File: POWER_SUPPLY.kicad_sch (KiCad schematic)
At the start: 70 parts, among them J1 Jack-DC, Q1 NTJD4401NT1G, Q2 NTJD4401NT1G, Q3 NTJD4401NT1G, U20 74LVC1G08, U21 74LVC1G08, U22 LM397, U23 74LVC1G17, U5 LM66100DCK, U6 LMR33640ADDA, U7 LMR33640ADDA

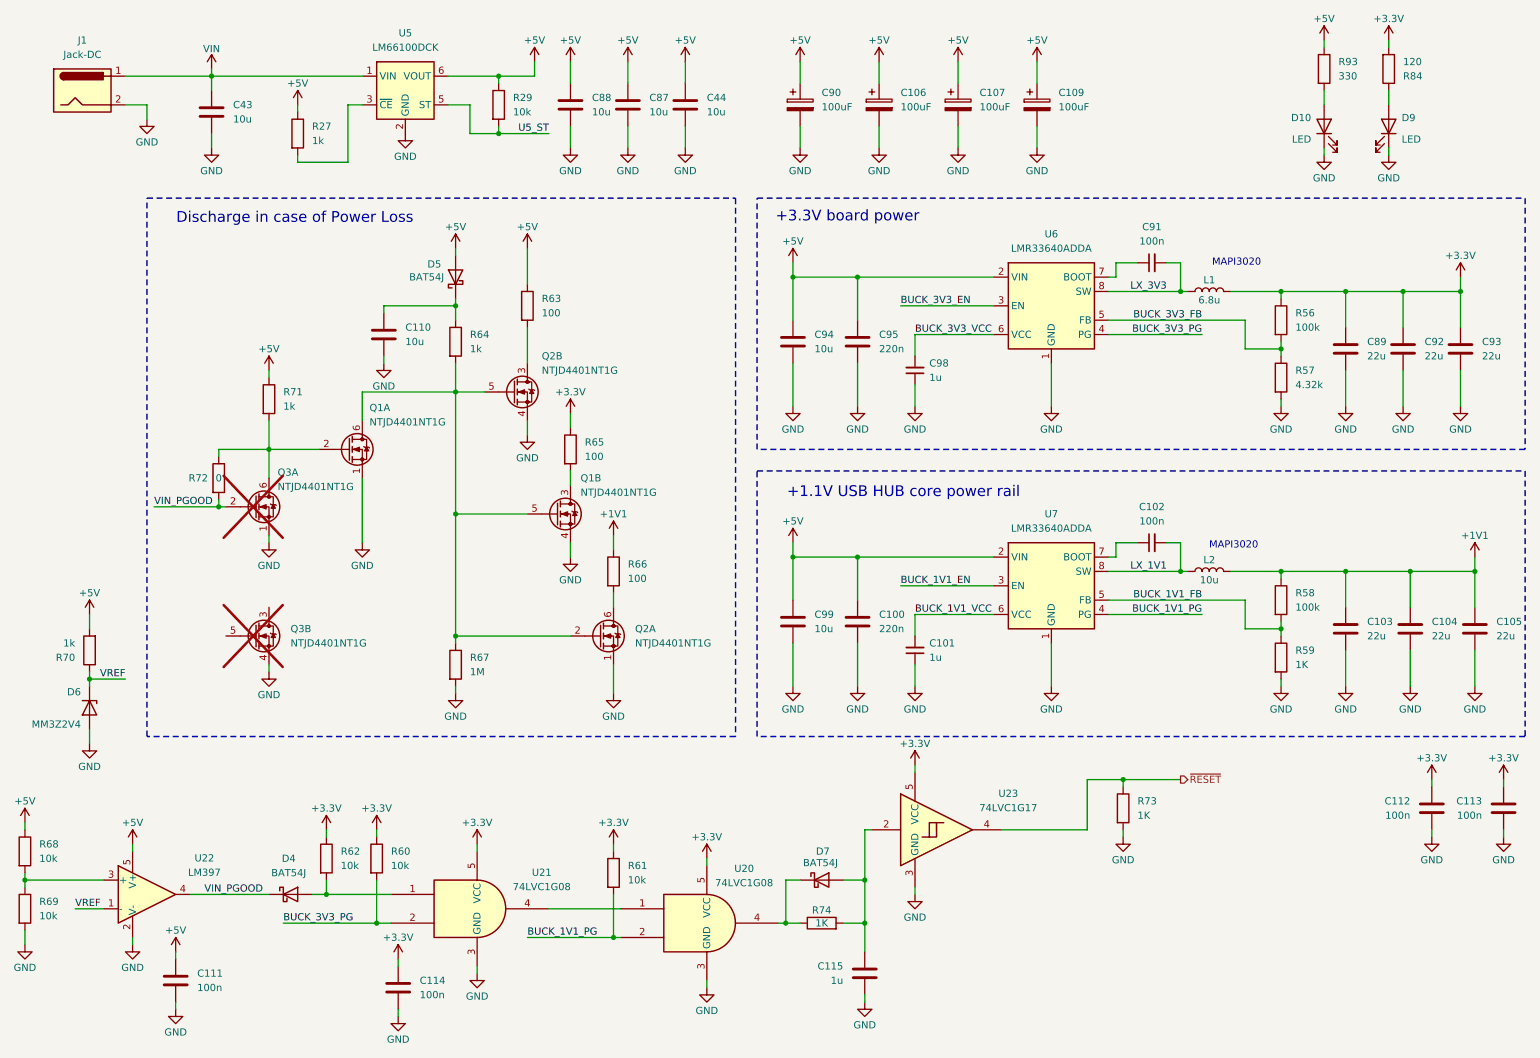
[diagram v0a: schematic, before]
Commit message: Powersequencing
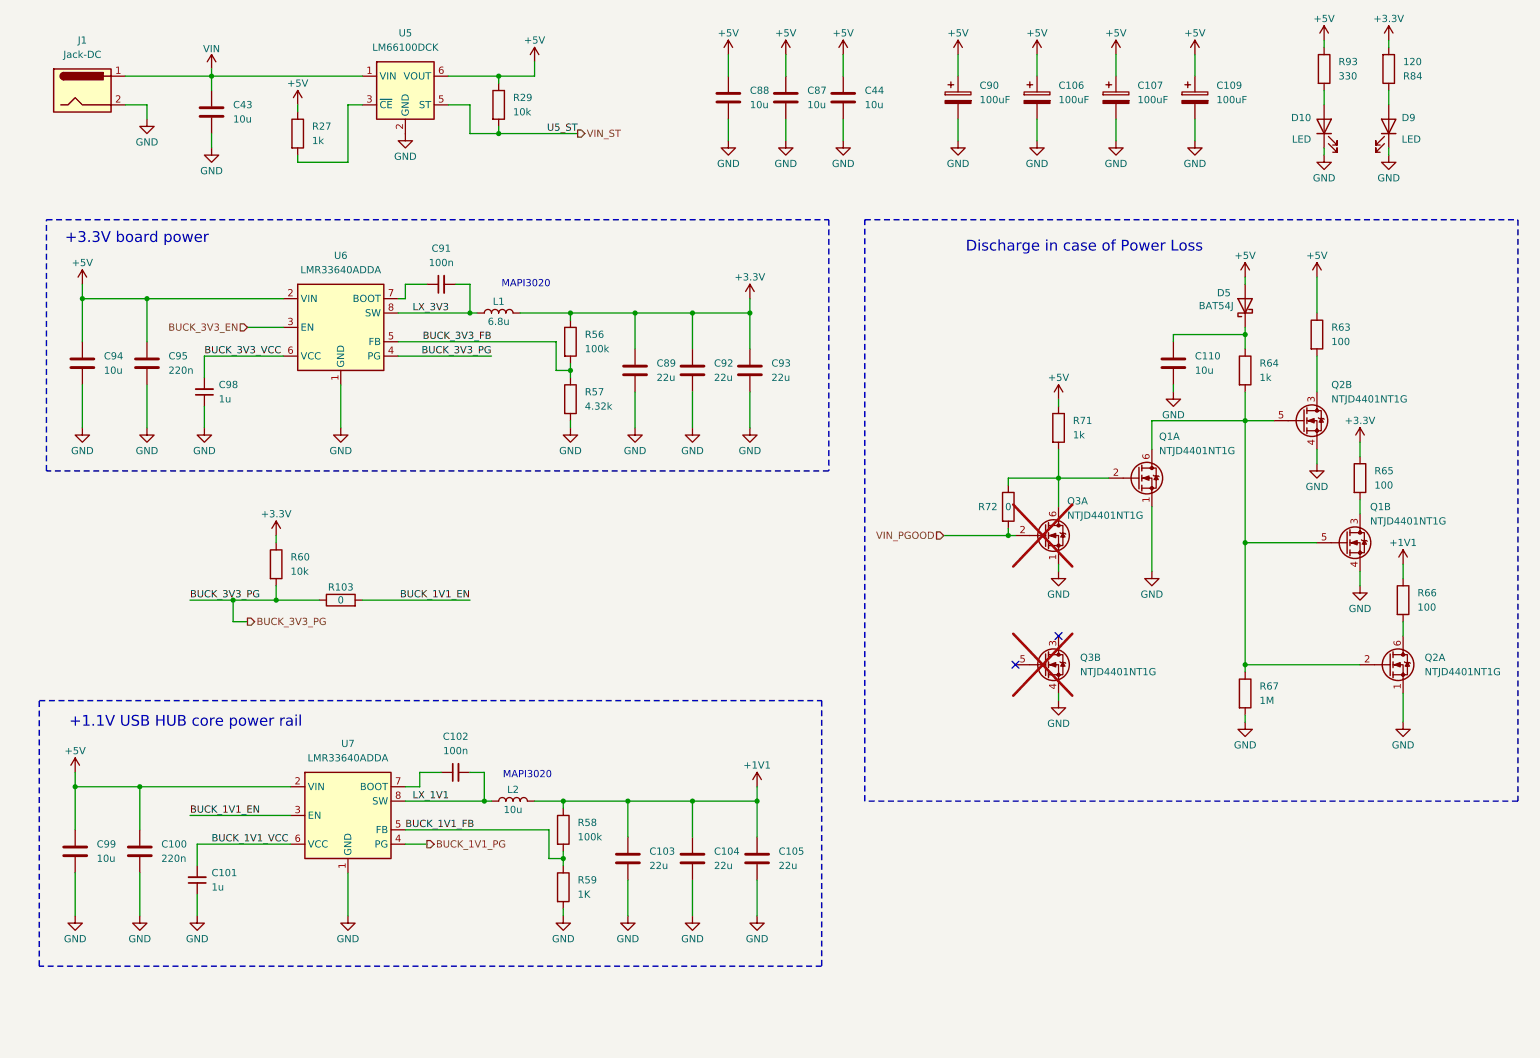
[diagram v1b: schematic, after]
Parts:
- removed C111, C112, C113, C114: 100n, 00_Capacitor:Cap_0402, symbol Device:C
- removed C115: 1u, 00_Capacitor:Cap_0402, symbol Device:C
- removed D4, D7: BAT54J, Diode_SMD:D_SOD-323F, symbol Diode:BAT54J
- removed D6: MM3Z2V4, Diode_SMD:D_SOD-323F, symbol Diode:MM3Zxx
- removed R61, R62, R68, R69: 10k, 00_Resistor:Res_0402, symbol Device:R
- removed R70: 1k, 00_Resistor:Res_0402, symbol Device:R
- removed R73, R74: 1K, 00_Capacitor:Cap_0402, symbol Device:R
- removed U20, U21: 74LVC1G08, Package_TO_SOT_SMD:SOT-23-5, symbol 74xGxx:74LVC1G08
- removed U22: LM397, Package_TO_SOT_SMD:SOT-23-5, symbol Comparator:LM397
- removed U23: 74LVC1G17, Package_TO_SOT_SMD:SOT-23-5, symbol 74xGxx:74LVC1G17
- added R103: 0, 00_Capacitor:Cap_0402, symbol Device:R
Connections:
- net BUCK_1V1_EN: now also R103.2
- net BUCK_3V3_PG: now also R103.1
- net U5_ST renamed VIN_ST
- no-connect marks 0 -> 2
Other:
- moved on the sheet: C100, C101, C102, C103, C104, C105, C106, C107, C109, C110, C44, C87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
